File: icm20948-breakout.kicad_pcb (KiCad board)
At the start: 2 copper layers, 11.6 x 20.8 mm, 14 parts, among them J1 Conn_01x04, Q1 BSS138, Q2 BSS138, U1 ICM-20948, U2 MIC5317-1.8xM5

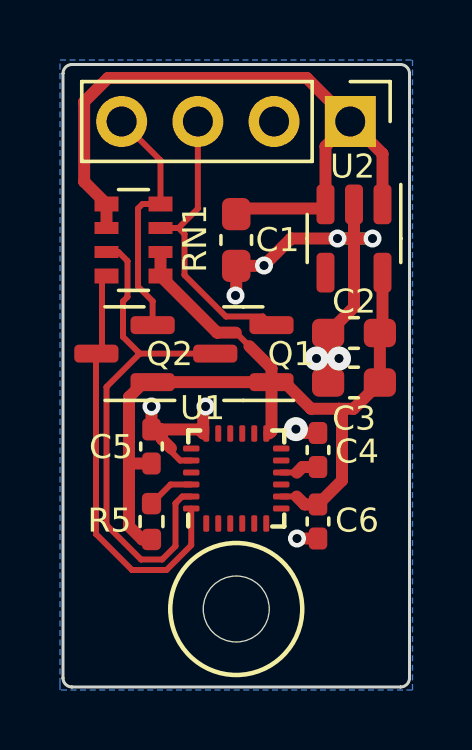
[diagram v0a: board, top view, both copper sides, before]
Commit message: A whole bunch of changes after speaking with Jon.
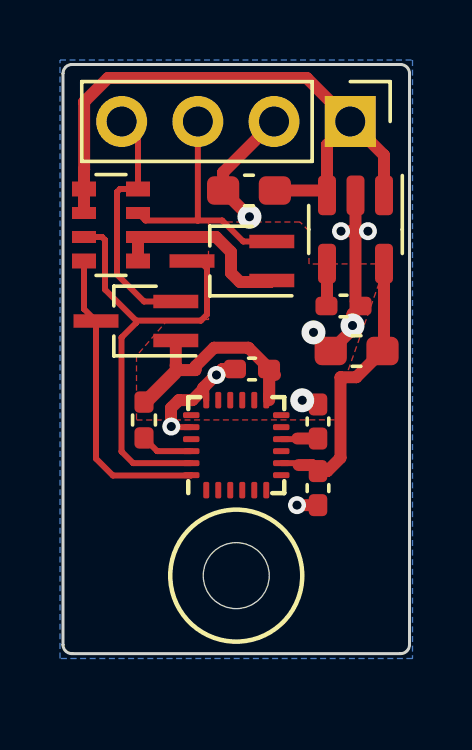
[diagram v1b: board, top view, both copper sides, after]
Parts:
- C2: value 100n -> 10n; footprint Capacitor_SMD:C_0603_1608Metric_Pad1.08x0.95mm_HandSolder -> Capacitor_SMD:C_0402_1005Metric_Pad0.74x0.62mm_HandSolder
- J1: footprint Connector_PinHeader_2.54mm:PinHeader_1x04_P2.54mm_Vertical -> local:PinHeader_1x04_P2.54mm_Vertical
- Q1, Q2: value BSS138 -> RJU003N03; footprint Package_TO_SOT_SMD:SOT-23 -> Package_TO_SOT_SMD:SOT-323_SC-70_Handsoldering
- U1: renamed from U2; value MIC5317-1.8xM5 -> RS3221-1.8
- moved C5 4.23 mm to (150.4, 100.1), turned to 180 degrees
- moved R5 3.39 mm to (146.8, 101.8), turned to -90 degrees
- moved Q1 3.11 mm to (149.7, 96.5)
- moved C1 1.70 mm to (150.3, 94.2), turned to 180 degrees
- moved Q2 1.15 mm to (146.5, 98.5)
- moved C6 1.11 mm to (152.6, 104.1)
- moved U2 1.11 mm to (149.9, 102.6)
- moved H1 1.11 mm to (149.9, 107.0)
- moved C3 1.05 mm to (153.9, 99.5)
- moved C2 0.97 mm to (153.4, 98.0), turned to 0 degrees
- moved C4 0.95 mm to (152.6, 101.8)
- moved RN1 0.90 mm to (145.7, 95.3)
- moved U1 0.30 mm to (153.8, 95.5)
- renumbered U1 to U2
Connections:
- C2 pad 1: +1V8 -> /psu/BP
- U1 pad 4: unconnected-(U2-NC-Pad4) (its old number) -> /psu/BP
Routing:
- net +1V8: track 31.9 -> 26.9 mm
- net GND: track 21.5 -> 17.5 mm, vias 10 -> 9
- net /SDA1_8: track 14.0 -> 10.2 mm
- net +3V3: track 23.7 -> 21.0 mm
- net /SCL1_8: track 17.9 -> 15.5 mm
- net /leveltrans/SCL: track 9.66 -> 8.15 mm
- net /psu/BP: track 0.00 -> 1.42 mm
- net /REGOUT: track 1.31 -> 1.93 mm
- added copper zone on F.Cu, net +1V8
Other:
- board size 11.6 x 20.8 mm -> 11.6 x 19.6 mm
- board text added: "v1.1a 6-Jan-2024"
- board text removed: "v1.0a 3-Jan-2024"

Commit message: Changes for v1.1b
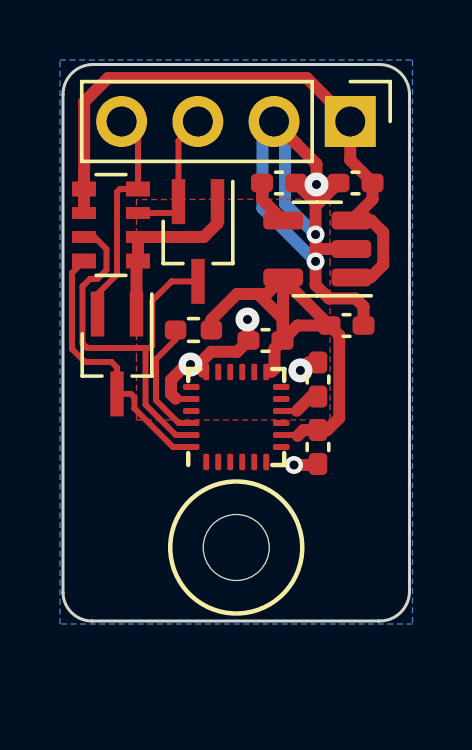
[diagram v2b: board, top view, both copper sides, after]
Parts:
- C1, C3: footprint Capacitor_SMD:C_0603_1608Metric_Pad1.08x0.95mm_HandSolder -> Capacitor_SMD:C_0402_1005Metric_Pad0.74x0.62mm_HandSolder
- Q1, Q2: footprint Package_TO_SOT_SMD:SOT-323_SC-70_Handsoldering -> local:SOT-323_SC-70_Handsoldering
- moved C2 4.63 mm to (151.3, 93.9)
- moved C1 3.56 mm to (153.8, 93.9)
- moved R5 3.42 mm to (148.4, 98.8), turned to 180 degrees
- moved U1 1.43 mm to (152.6, 96.1), turned to 180 degrees
- moved C4 1.40 mm to (152.6, 100.5)
- moved C6 1.37 mm to (152.6, 102.7)
- moved Q1 1.30 mm to (148.6, 95.8), turned to -90 degrees
- moved Q2 1.27 mm to (145.9, 99.6), turned to -90 degrees
- moved C5 1.05 mm to (150.8, 99.2)
- moved H1 0.94 mm to (149.9, 106.0)
- moved U2 0.94 mm to (149.9, 101.7)
- moved C3 0.91 mm to (153.6, 98.7), turned to 0 degrees
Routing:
- net GND: track 17.5 -> 30.8 mm, vias 9 -> 7
- net /leveltrans/SCL: track 8.15 -> 4.75 mm
- net +1V8: track 26.9 -> 24.1 mm
- net /CS: track 1.76 -> 4.10 mm
- net /SCL1_8: track 15.5 -> 14.1 mm
- net /SDA1_8: track 10.2 -> 9.18 mm
- net /leveltrans/SDA: track 8.30 -> 7.56 mm
- net /REGOUT: track 1.93 -> 1.42 mm
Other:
- board size 11.6 x 19.6 mm -> 11.6 x 18.5 mm
- board text added: "v1.1b 6-Jan-2024"
- board text removed: "v1.1a 6-Jan-2024"
